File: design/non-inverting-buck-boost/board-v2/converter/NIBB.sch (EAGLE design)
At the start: 10 parts

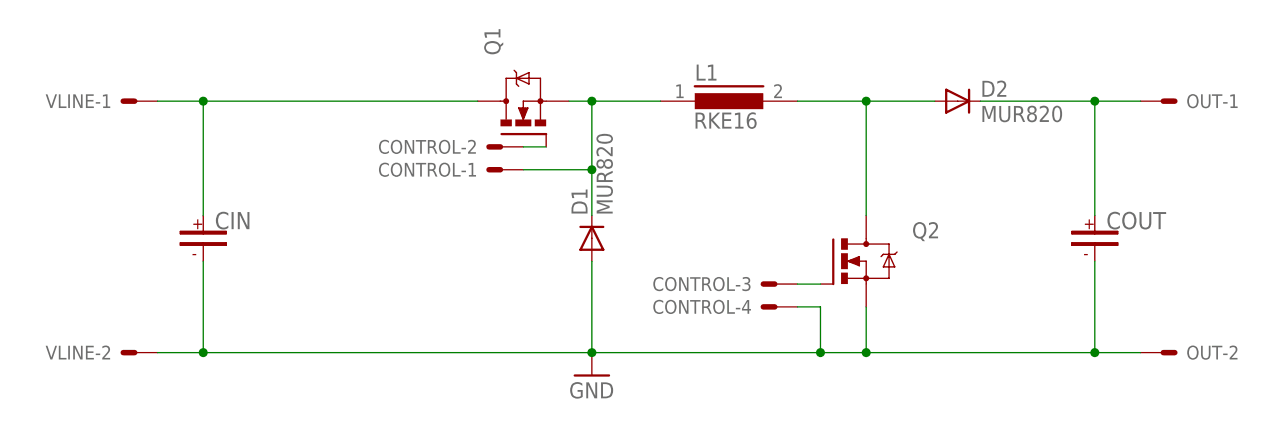
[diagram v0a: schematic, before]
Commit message: revert commit
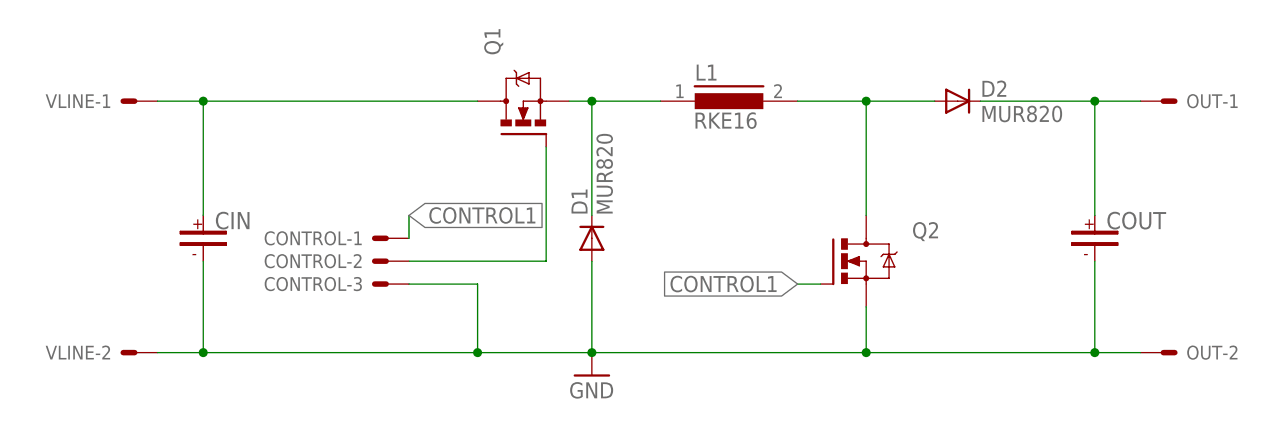
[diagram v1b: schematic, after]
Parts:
- CONTROL: value 22-23-2041 -> 22-23-2031; device con-molex:22-23-2041 -> con-molex:22-23-2031
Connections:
- net N$4 renamed CONTROL2
- removed net N$5: CONTROL-3.S, Q2.G
- new net CONTROL1: CONTROL-1.S, Q2.G
- net GND: now also CONTROL-3.S; no longer CONTROL-4.S
- net N$1: no longer CONTROL-1.S
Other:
- moved on the sheet: CONTROL-1, CONTROL-2, CONTROL-3
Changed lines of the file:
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@@
 <setting verticaltext="up"/>
 </settings>
-<grid distance="0.1" unitdist="inch" unit="inch" style="lines" multiple="1" display="no" altdistance="0.01" altunitdist="inch" altunit="inch"/>
+<grid distance="0.1" unitdist="inch" unit="inch" style="lines" multiple="1" display="yes" altdistance="0.01" altunitdist="inch" altunit="inch"/>
 <layers>
 <layer number="1" name="Top" color="4" fill="1" visible="no" active="no"/>
@@
 <part name="Q2" library="felippe" deviceset="IRF640" device=""/>
 <part name="GND1" library="supply1" deviceset="GND" device=""/>
+<part name="CONTROL" library="con-molex" deviceset="22-23-2031" device=""/>
 <part name="CIN" library="capacitor" deviceset="CAPP-U" device="F"/>
-<part name="CONTROL" library="con-molex" deviceset="22-23-2041" device=""/>
 </parts>
 <sheets>
@@
 <instance part="Q2" gate="G$1" x="53.34" y="45.72"/>
 <instance part="GND1" gate="1" x="25.4" y="33.02"/>
+<instance part="CONTROL" gate="-1" x="2.54" y="48.26" smashed="yes" rot="R180">
+<attribute name="NAME" x="0" y="49.022" size="1.524" layer="95" rot="R180"/>
+</instance>
+<instance part="CONTROL" gate="-2" x="2.54" y="45.72" rot="R180"/>
+<instance part="CONTROL" gate="-3" x="2.54" y="43.18" rot="R180"/>
 <instance part="CIN" gate="G$1" x="-17.78" y="48.26"/>
-<instance part="CONTROL" gate="-1" x="15.24" y="55.88" smashed="yes" rot="R180">
-<attribute name="NAME" x="12.7" y="56.642" size="1.524" layer="95" rot="R180"/>
-</instance>
-<instance part="CONTROL" gate="-2" x="15.24" y="58.42" rot="R180"/>
-<instance part="CONTROL" gate="-3" x="45.72" y="43.18" rot="R180"/>
-<instance part="CONTROL" gate="-4" x="45.72" y="40.64" rot="R180"/>
 </instances>
 <busses>
@@
 </segment>
 </net>
+<net name="CONTROL1" class="0">
+<segment>
+<pinref part="Q2" gate="G$1" pin="G"/>
+<wire x1="50.8" y1="43.18" x2="48.26" y2="43.18" width="0.1524" layer="91"/>
+<label x="48.26" y="43.18" size="1.778" layer="95" rot="R180" xref="yes"/>
+</segment>
+<segment>
+<pinref part="CONTROL" gate="-1" pin="S"/>
+<wire x1="5.08" y1="48.26" x2="5.08" y2="50.8" width="0.1524" layer="91"/>
+<label x="5.08" y="50.8" size="1.778" layer="95" xref="yes"/>
+</segment>
+</net>
 <net name="N$7" class="0">
 <segment>
@@
 <pinref part="D1" gate="1" pin="C"/>
 <wire x1="25.4" y1="63.5" x2="33.02" y2="63.5" width="0.1524" layer="91"/>
+<wire x1="25.4" y1="50.8" x2="25.4" y2="63.5" width="0.1524" layer="91"/>
 <junction x="25.4" y="63.5"/>
 <pinref part="Q1" gate="G$1" pin="S"/>
-<wire x1="25.4" y1="50.8" x2="25.4" y2="55.88" width="0.1524" layer="91"/>
-<pinref part="CONTROL" gate="-1" pin="S"/>
-<wire x1="25.4" y1="55.88" x2="25.4" y2="63.5" width="0.1524" layer="91"/>
-<wire x1="17.78" y1="55.88" x2="25.4" y2="55.88" width="0.1524" layer="91"/>
-<junction x="25.4" y="55.88"/>
 </segment>
 </net>
@@
 <wire x1="-22.86" y1="35.56" x2="-17.78" y2="35.56" width="0.1524" layer="91"/>
 <pinref part="COUT" gate="G$1" pin="-"/>
-<wire x1="-17.78" y1="35.56" x2="25.4" y2="35.56" width="0.1524" layer="91"/>
-<wire x1="25.4" y1="35.56" x2="50.8" y2="35.56" width="0.1524" layer="91"/>
-<wire x1="50.8" y1="35.56" x2="55.88" y2="35.56" width="0.1524" layer="91"/>
+<wire x1="-17.78" y1="35.56" x2="12.7" y2="35.56" width="0.1524" layer="91"/>
+<wire x1="12.7" y1="35.56" x2="25.4" y2="35.56" width="0.1524" layer="91"/>
+<wire x1="25.4" y1="35.56" x2="55.88" y2="35.56" width="0.1524" layer="91"/>
 <wire x1="81.28" y1="45.72" x2="81.28" y2="35.56" width="0.1524" layer="91"/>
 <wire x1="81.28" y1="35.56" x2="55.88" y2="35.56" width="0.1524" layer="91"/>
@@
 <pinref part="Q2" gate="G$1" pin="S"/>
 <pinref part="GND1" gate="1" pin="GND"/>
+<pinref part="CONTROL" gate="-3" pin="S"/>
+<wire x1="5.08" y1="43.18" x2="12.7" y2="43.18" width="0.1524" layer="91"/>
+<wire x1="12.7" y1="43.18" x2="12.7" y2="35.56" width="0.1524" layer="91"/>
+<junction x="12.7" y="35.56"/>
 <pinref part="CIN" gate="G$1" pin="-"/>
 <wire x1="-17.78" y1="45.72" x2="-17.78" y2="35.56" width="0.1524" layer="91"/>
 <junction x="-17.78" y="35.56"/>
-<wire x1="50.8" y1="40.64" x2="50.8" y2="35.56" width="0.1524" layer="91"/>
-<junction x="50.8" y="35.56"/>
-<pinref part="CONTROL" gate="-4" pin="S"/>
-<wire x1="48.26" y1="40.64" x2="50.8" y2="40.64" width="0.1524" layer="91"/>
-</segment>
-</net>
-<net name="N$4" class="0">
+</segment>
+</net>
+<net name="CONTROL2" class="0">
 <segment>
 <pinref part="CONTROL" gate="-2" pin="S"/>
+<wire x1="5.08" y1="45.72" x2="20.32" y2="45.72" width="0.1524" layer="91"/>
 <pinref part="Q1" gate="G$1" pin="G"/>
-<wire x1="17.78" y1="58.42" x2="20.32" y2="58.42" width="0.1524" layer="91"/>
-</segment>
-</net>
-<net name="N$5" class="0">
-<segment>
-<pinref part="CONTROL" gate="-3" pin="S"/>
-<pinref part="Q2" gate="G$1" pin="G"/>
-<wire x1="48.26" y1="43.18" x2="50.8" y2="43.18" width="0.1524" layer="91"/>
-</segment>
-</net>
+<wire x1="20.32" y1="45.72" x2="20.32" y2="58.42" width="0.1524" layer="91"/>
+</segment>
+</net>
